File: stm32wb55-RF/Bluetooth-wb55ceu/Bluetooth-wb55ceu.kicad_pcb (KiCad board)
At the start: 4 copper layers, 50.1 x 39.9 mm, 48 parts, among them J1 USB_C_Receptacle_USB2.0_16P, J2 Conn_Coaxial, J3 Conn_01x04_Pin, J4 Conn_02x05_Odd_Even, SW1 SW_Push, U1 LM1117MP-3.3, U2 USBLC6-2SC6, U3 STM32WB55CEUx, Y1 32KHz, Y2 12MHz

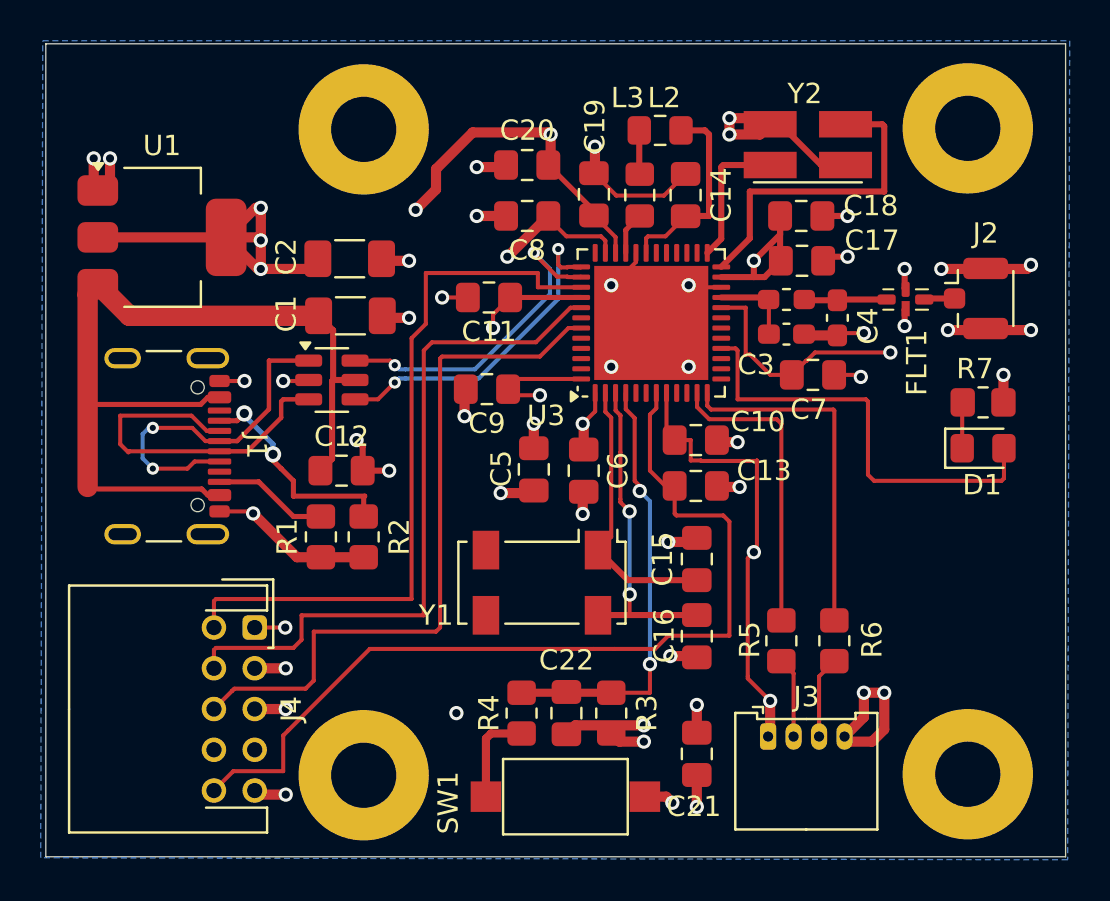
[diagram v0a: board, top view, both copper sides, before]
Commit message: Folder updated
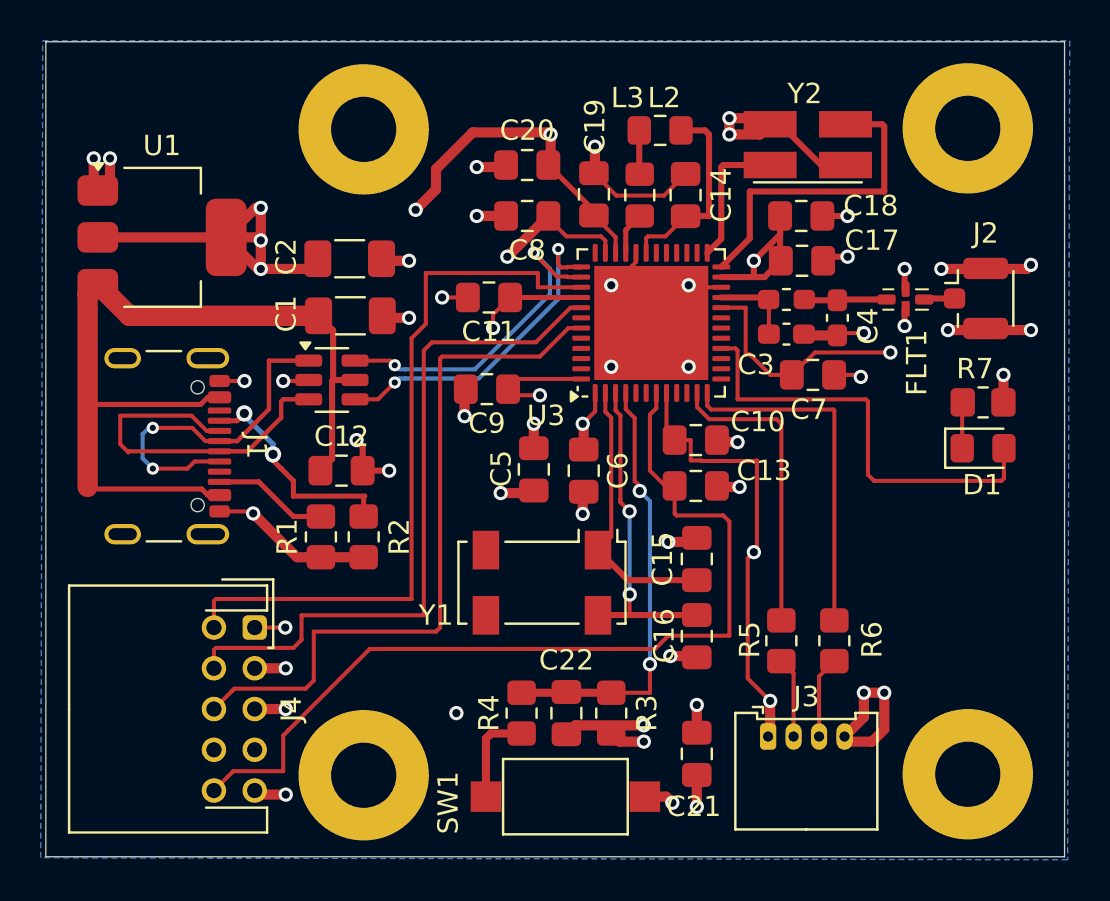
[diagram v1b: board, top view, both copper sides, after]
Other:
- board size 50.1 x 39.9 mm -> 50 x 40 mm
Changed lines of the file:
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@@
 	)
 	(gr_line
-		(start 252.9 104.45)
+		(start 252.85 104.45)
 		(end 202.85 104.45)
 		(stroke
@@
 	(gr_line
 		(start 202.85 104.45)
-		(end 202.85 64.55)
+		(end 202.85 64.45)
 		(stroke
 			(width 0.05)
@@
 	)
 	(gr_line
-		(start 252.9 64.55)
-		(end 252.9 104.45)
+		(start 252.85 64.45)
+		(end 252.85 104.45)
 		(stroke
 			(width 0.05)
@@
 	)
 	(gr_line
-		(start 202.85 64.55)
-		(end 252.9 64.55)
+		(start 202.85 64.45)
+		(end 252.85 64.45)
 		(stroke
 			(width 0.05)
